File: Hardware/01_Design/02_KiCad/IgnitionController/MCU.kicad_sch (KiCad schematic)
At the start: 0 parts

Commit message: MCU sheet Initial commit
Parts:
- added C16, C17, C18, C19: 12p, symbol Device:C_Small
- added C20, C22, C24, C26, C28, C30, C32, C34, C36: 0.1u, symbol Device:C_Small
- added C21, C23, C25, C27, C29, C31, C33, C35: 1u, symbol Device:C_Small
- added D1, D2, D3, D4, D5: RED, symbol Device:LED
- added R1, R4: 10k, symbol Device:R_Small
- added R2: 510R, symbol Device:R_Small
- added R3: 0R, symbol Device:R_Small
- added R40, R41, R42, R43, R44: 470R, symbol Device:R_Small
- added TP10: Cyl1_TP, symbol Connector:TestPoint
- added TP11: Cyl2_TP, symbol Connector:TestPoint
- added TP12: Sig1_TP, symbol Connector:TestPoint
- added TP13: Sig2_TP, symbol Connector:TestPoint
- added U12: STM32F407VGTx, Package_QFP:LQFP-100_14x14mm_P0.5mm, symbol Library_sym.pretty:STM32F407VGTx
- added Y2: 32.768kHz, symbol Device:Crystal_Small
- added Y3: 8MHz, symbol Device:Crystal_Small
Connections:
- new net: C18.2, U12.12 (PH0), Y3.2
- new net: C17.1, U12.8 (PC14), Y2.1
- new net: C16.2, U12.9 (PC15), Y2.2
- new net: R44.1, U12.62 (PD15)
- new net: D5.2 (A), R44.2
- new net: D2.2 (A), R41.2
- new net: D4.2 (A), R43.2
- new net: C19.1, U12.13 (PH1), Y3.1
- new net: C20.1, R4.2, U12.14 (NRST)
- new net: R1.2, R2.1, U12.94 (BOOT0)
- new net: D3.2 (A), R42.2
- new net: D1.2 (A), R40.2
- new net: R2.2, R3.1
- new net CAN_RXD: U12.95 (PB8)
- new net CAN_TXD: U12.96 (PB9)
- new net Cylinder1Out_Pin: R41.1, TP10.1, U12.53 (PB14)
- new net Cylinder2Out_Pin: R40.1, TP11.1, U12.52 (PB13)
- new net GND: C16.1, C17.2, C18.1, C19.2, C20.2, C21.2, C22.2, C23.2, C24.2, C25.2, C26.2, C27.2, C28.2, C29.2, C30.2, C31.2, C32.2, C33.2, C34.2, C35.2, C36.2, D1.1 (K), D2.1 (K), D3.1 (K), D4.1 (K), D5.1 (K), R3.2, U12.10 (VSS), U12.20 (VSSA), U12.27 (VSS), U12.74 (VSS), U12.99 (VSS)
- new net I2C_SCL: U12.92 (PB6)
- new net I2C_SDA: U12.93 (PB7)
- new net MCU_SPI_CS: U12.67 (PA8)
- new net MCU_SPI_MISO: U12.31 (PA6)
- new net MCU_SPI_MOSI: U12.32 (PA7)
- new net MCU_SPI_SCK: U12.30 (PA5)
- new net OE_PIN: U12.68 (PA9)
- new net SWCLK_Pin: U12.76 (PA14)
- new net SWDIO_Pin: U12.72 (PA13)
- new net Signal1_Pin: R42.1, TP12.1, U12.29 (PA4)
- new net Signal2_Pin: TP13.1, U12.41 (PE10)
- new net UART_RX: U12.79 (PC11)
- new net UART_TX: U12.78 (PC10)
- new net VMCU: C21.1, C22.1, C23.1, C24.1, C25.1, C26.1, C27.1, C28.1, C29.1, C30.1, C31.1, C32.1, C33.1, C34.1, C35.1, C36.1, R1.1, R4.1, U12.100 (VDD), U12.11 (VDD), U12.19 (VDD), U12.21 (VREF+), U12.22 (VDDA), U12.28 (VDD), U12.50 (VDD), U12.75 (VDD)

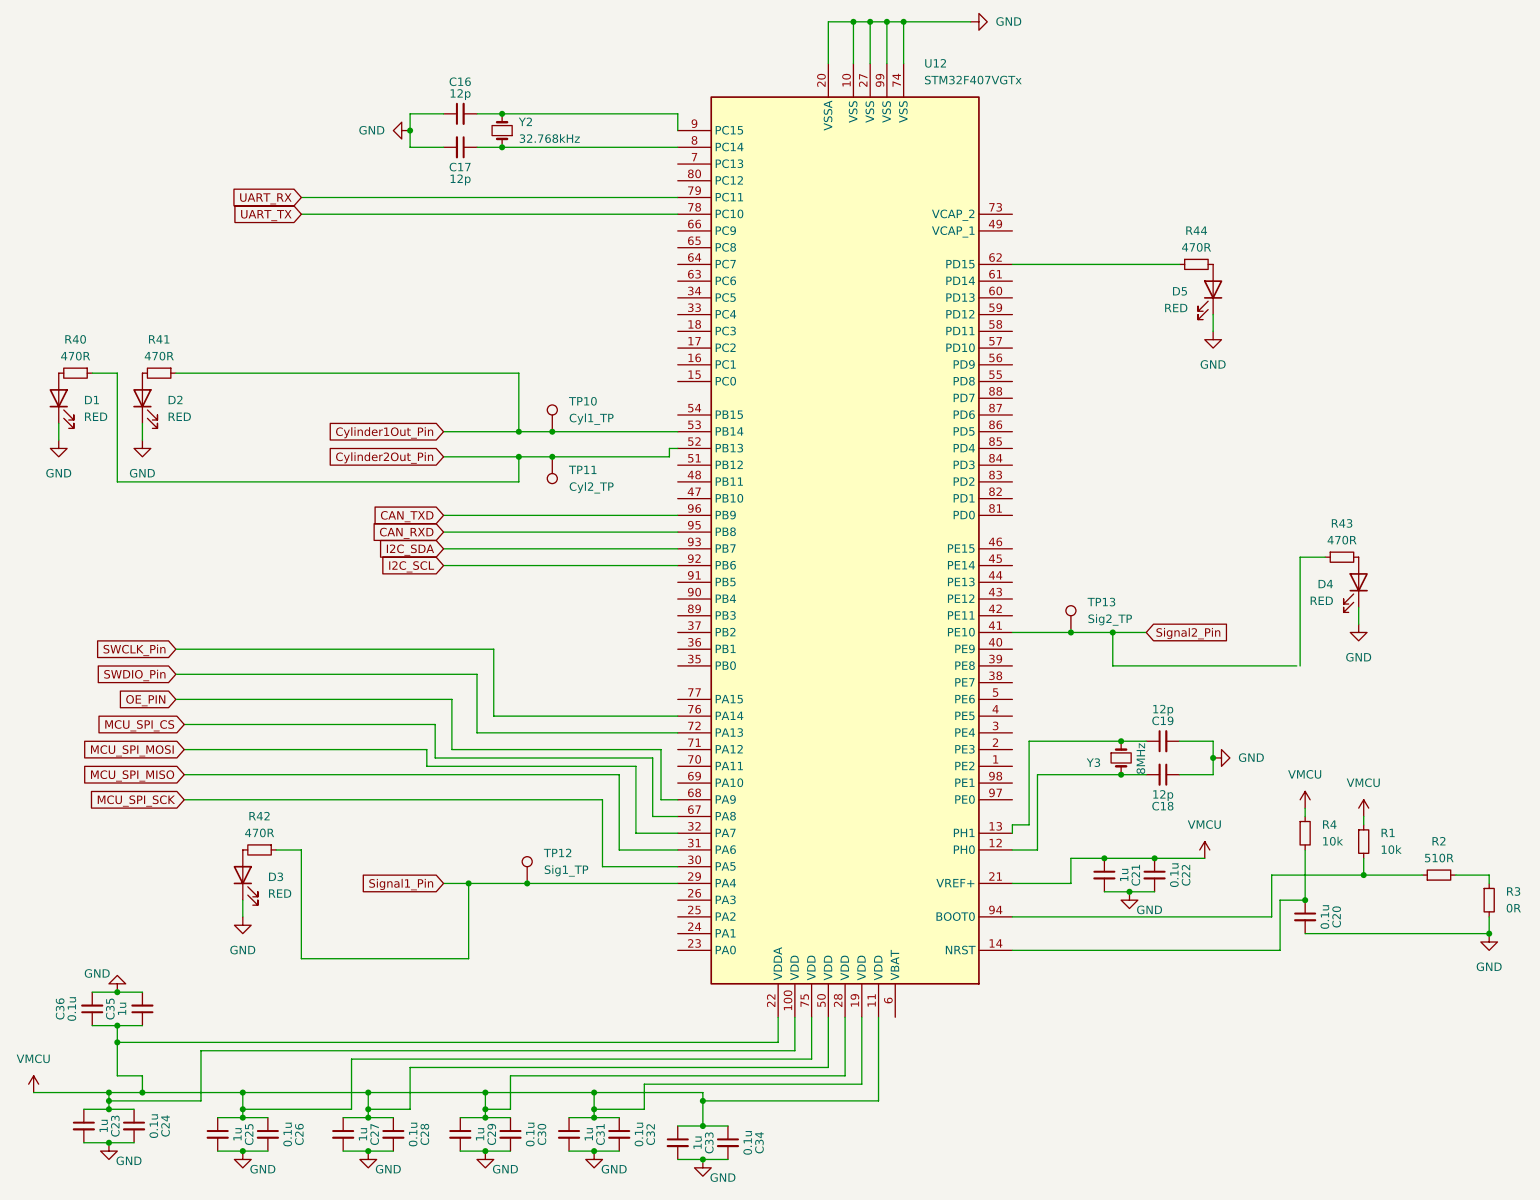
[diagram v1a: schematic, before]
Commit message: Peripherals Update
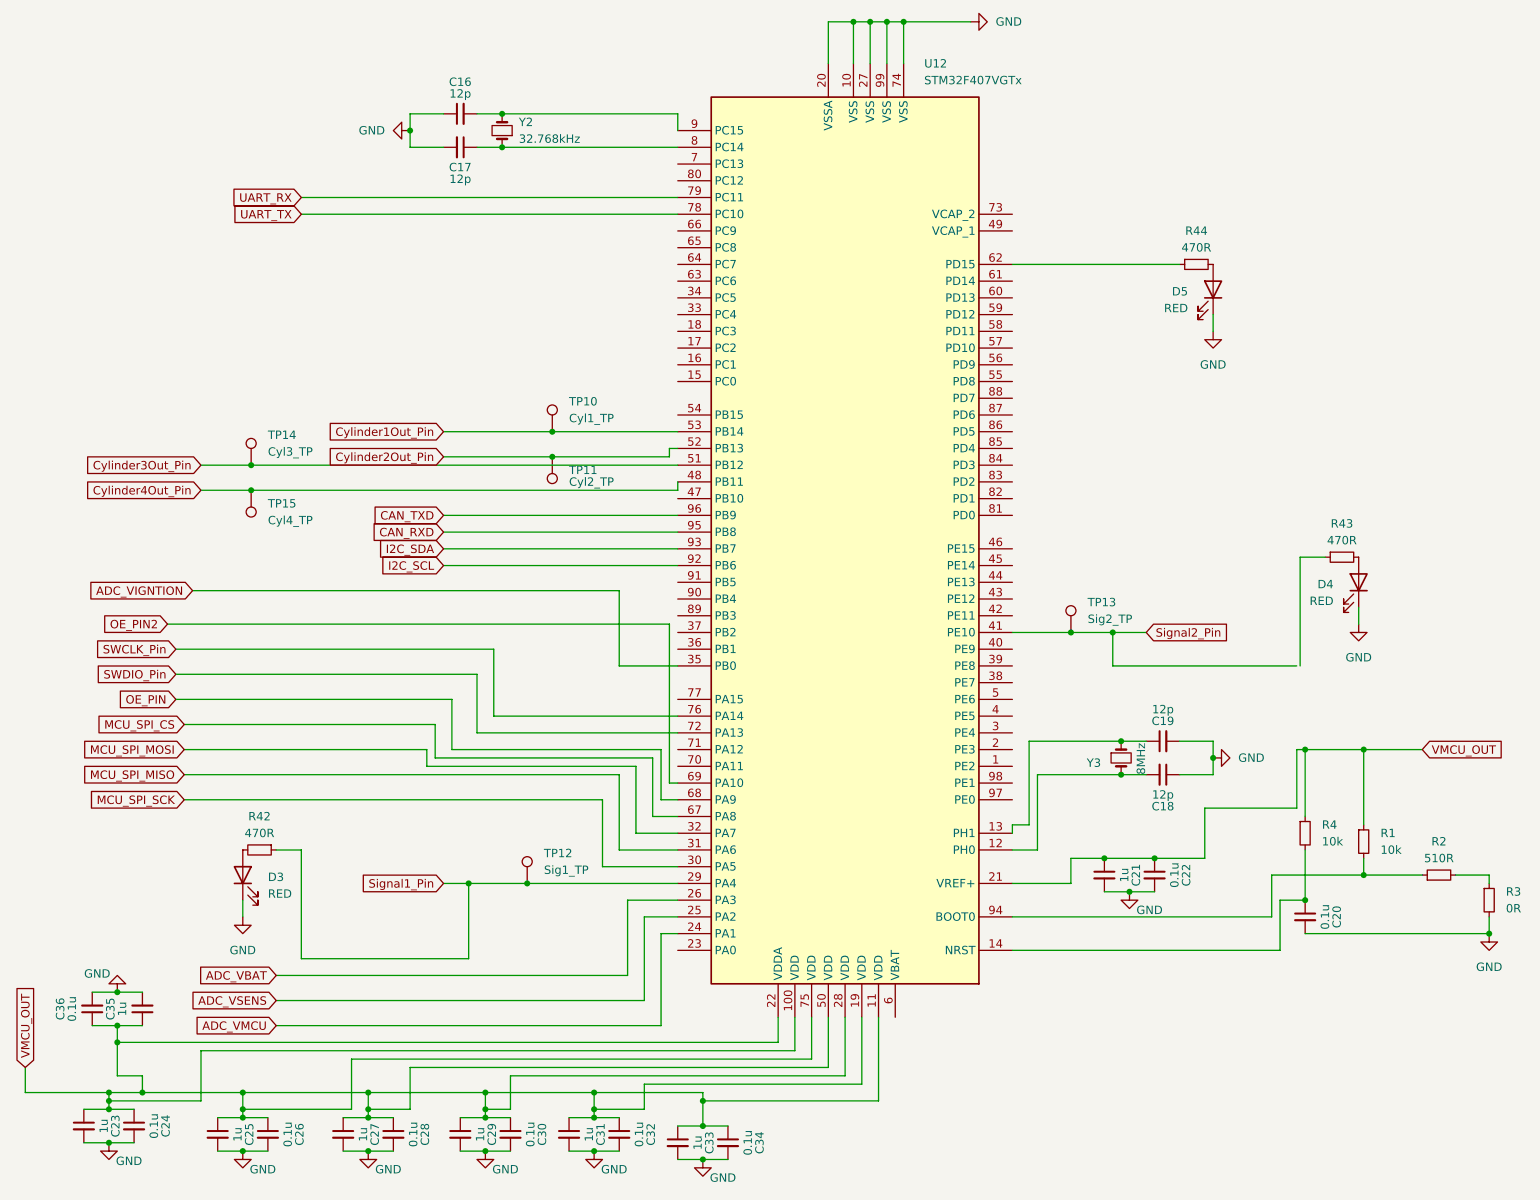
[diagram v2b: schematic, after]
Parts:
- removed D1, D2: RED, symbol Device:LED
- removed R40, R41: 470R, symbol Device:R_Small
- added TP14: Cyl3_TP, symbol Connector:TestPoint
- added TP15: Cyl4_TP, symbol Connector:TestPoint
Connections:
- net ADC_VMCU: now reaches U12.24 (PA1)
- net ADC_VSENS: now reaches U12.25 (PA2)
- net ADC_VBAT: now reaches U12.26 (PA3)
- net ADC_VIGNTION: now reaches U12.35 (PB0)
- net Cylinder4Out_Pin: now reaches U12.48 (PB11)
- net Cylinder4Out_Pin: now also TP15.1
- net Cylinder3Out_Pin: now reaches U12.51 (PB12)
- net Cylinder3Out_Pin: now also TP14.1
- net OE_PIN2: now reaches U12.69 (PA10)
- net VMCU renamed VMCU_OUT
